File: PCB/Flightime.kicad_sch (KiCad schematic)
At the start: 27 parts, among them J1 JST_02, J2 JST_02, J3 JST_02, J4 JST_02, J5 Conn_01x02_Pin, J6 Conn_01x02_Pin, Q1 AO3400A, Q2 AO3400A, Q3 AO3400A, Q4 AO3400A, SW1 SW_Nidec_CAS-120A1, U1 XIAO-ESP32-S3-SMD, U2 GY-521

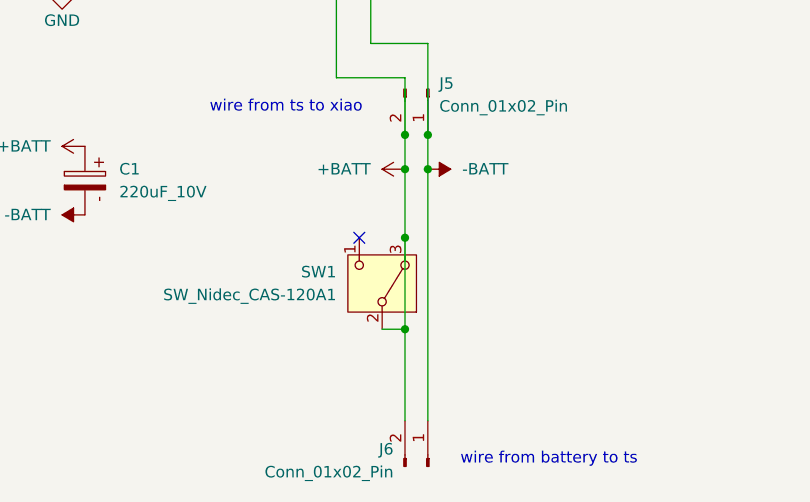
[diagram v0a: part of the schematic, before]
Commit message: reorientazted s3
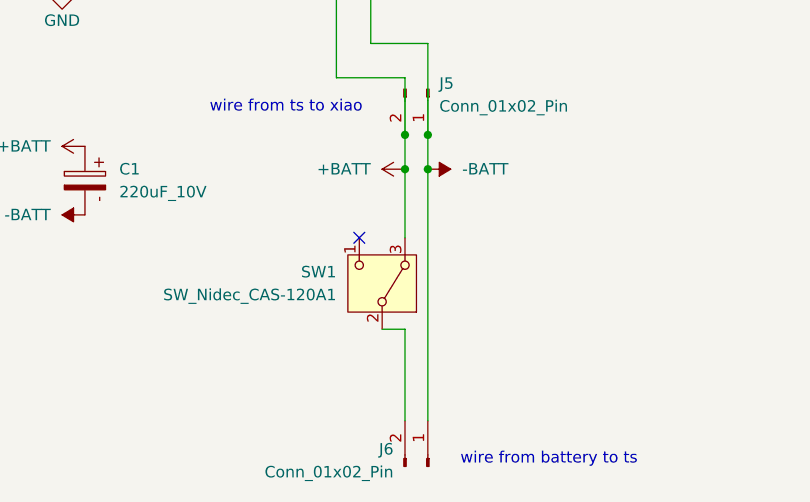
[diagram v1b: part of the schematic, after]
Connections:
- net +BATT: no longer J6.2 (Pin_2), SW1.2 (B)
- new net: J6.2 (Pin_2), SW1.2 (B)
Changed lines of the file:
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@@
-	)
-	(junction
-		(at 153.67 132.08)
-		(diameter 0)
-		(color 0 0 0 0)
 	)
 	(junction
@@
 	(junction
 		(at 82.55 93.98)
-		(diameter 0)
-		(color 0 0 0 0)
-	)
-	(junction
-		(at 153.67 142.24)
 		(diameter 0)
 		(color 0 0 0 0)
@@
 		)
 		(stroke
-			(width 0)
-			(type default)
-		)
-	)
-	(wire
-		(pts
-			(xy 153.67 132.08) (xy 153.67 142.24)
-		)
-		(stroke
